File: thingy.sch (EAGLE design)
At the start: 20 parts, among them IC1 MCP6001T-I/OT, IC2 MAX9812LEXT+T, IC3 ESP-12, IC4 ADXL345BCCZ, J1 Interface, Q1 Electret Mic

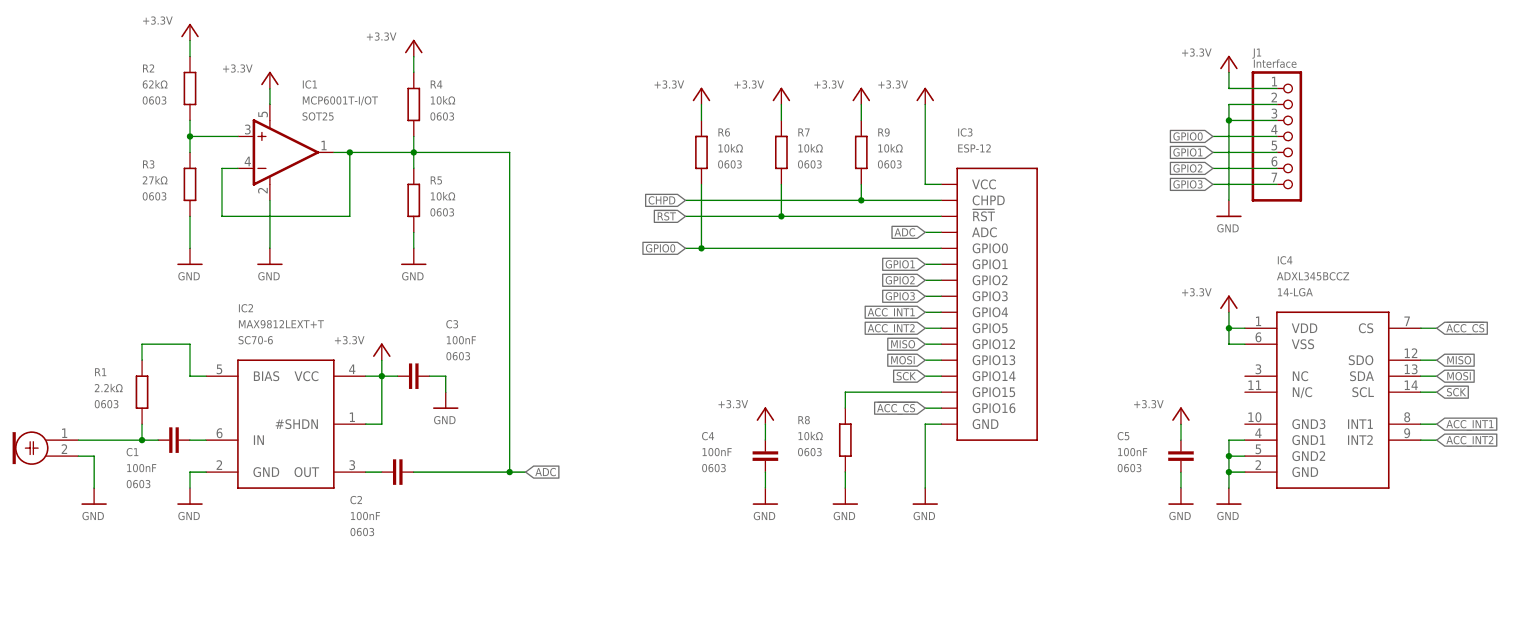
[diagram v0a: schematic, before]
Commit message: foo
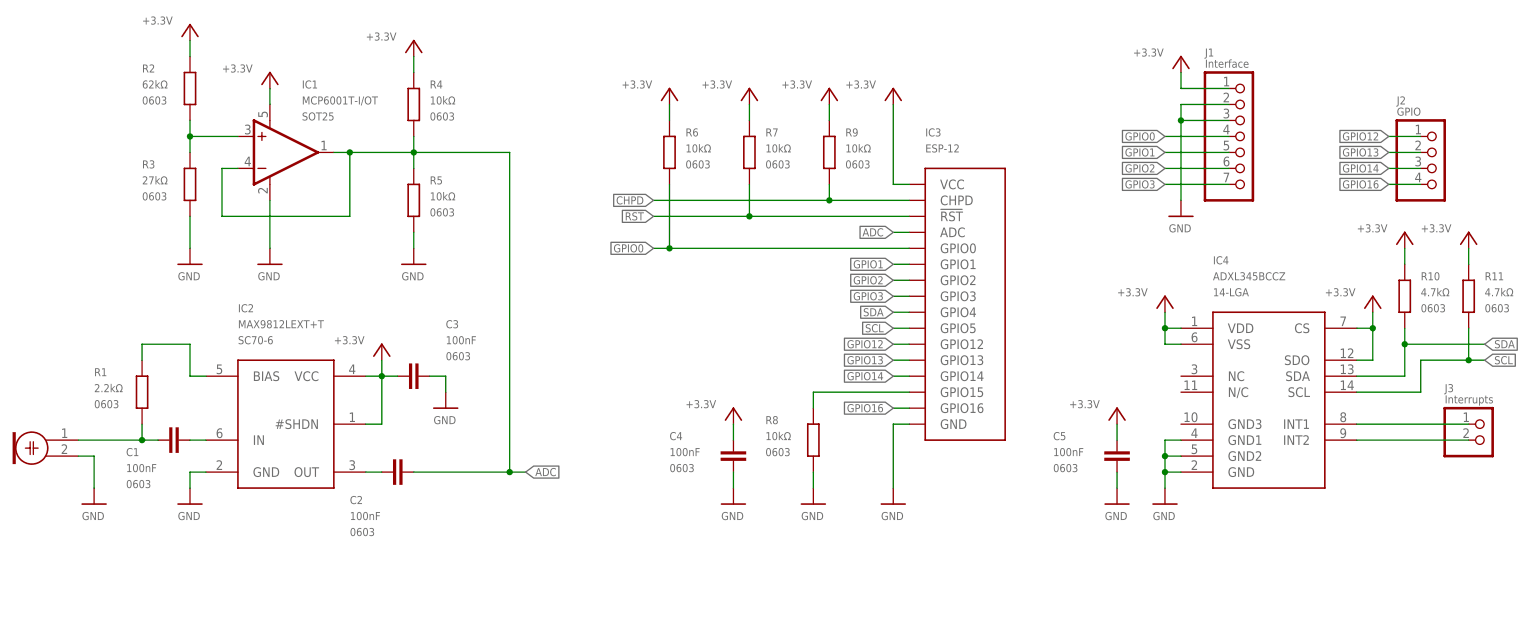
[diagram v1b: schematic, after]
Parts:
- added J2: GPIO, pinhead:PINHD-1X4
- added J3: Interrupts, pinhead:PINHD-1X2
- added R10, R11: 4.7kΩ, freetronics-luke:R0603
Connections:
- removed net !ACC_CS: IC3.GPIO16, IC4.CS
- removed net MISO: IC3.GPIO12, IC4.SDO
- removed net MOSI: IC3.GPIO13, IC4.SDA
- removed net SCK: IC3.GPIO14, IC4.SCL
- new net GPIO12: IC3.GPIO12, J2.1
- new net GPIO13: IC3.GPIO13, J2.2
- new net GPIO14: IC3.GPIO14, J2.3
- new net GPIO16: IC3.GPIO16, J2.4
- new net SCL: IC3.GPIO5, IC4.SCL, R11.1
- new net SDA: IC3.GPIO4, IC4.SDA, R10.1
- net +3.3V: now also IC4.CS, IC4.SDO, R10.2, R11.2
- net ACC_INT1: now also J3.1; no longer IC3.GPIO4
- net ACC_INT2: now also J3.2; no longer IC3.GPIO5
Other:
- note removed: "Could use I2C instead if you like."
- moved on the sheet: C4, C5, IC3, IC4, J1, R6, R7, R8, R9

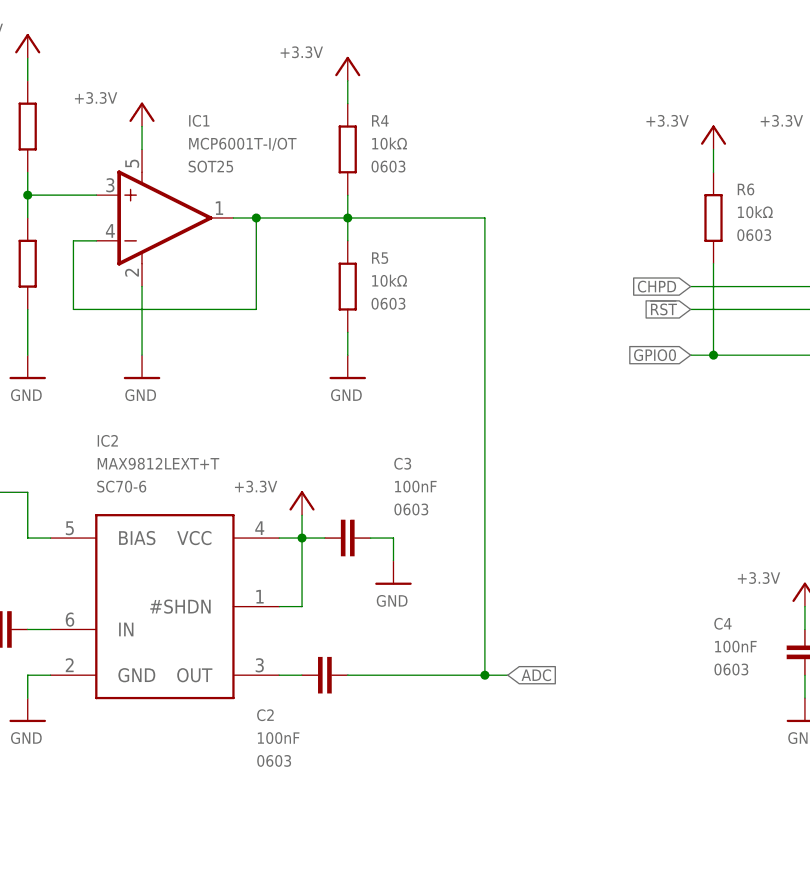
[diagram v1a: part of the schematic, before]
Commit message: foo
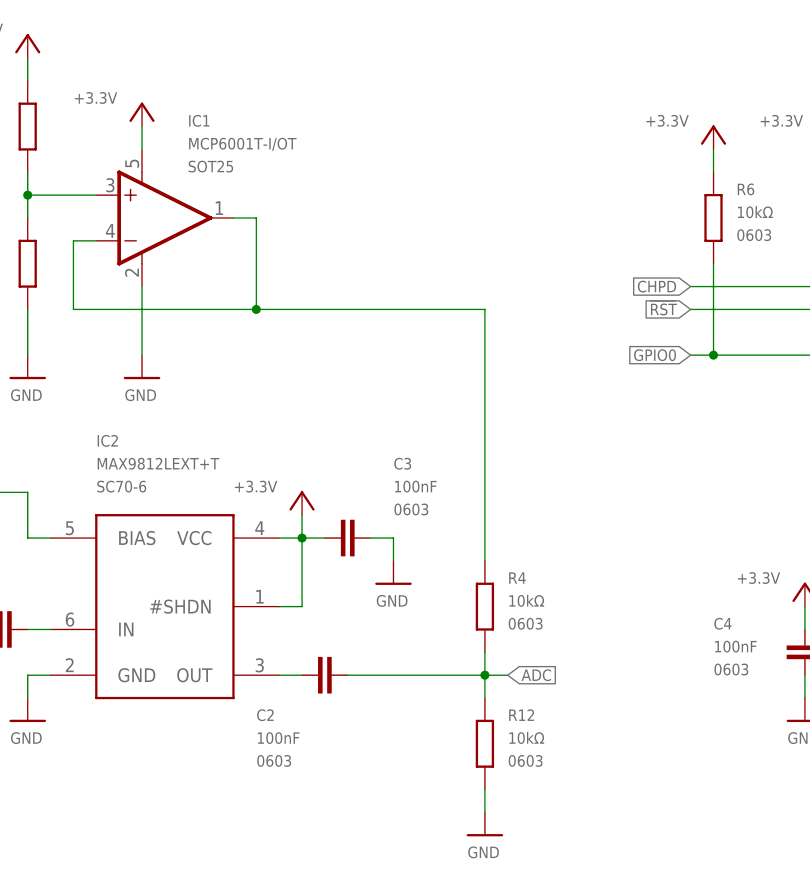
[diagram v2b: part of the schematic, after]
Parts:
- removed R5: 10kΩ, freetronics-luke:R0603
- added R12: 10kΩ, freetronics-luke:R0603
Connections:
- new net N$1: IC1.-IN, IC1.OUT, R4.2
- net +3.3V: no longer R4.2
- net ADC: now also R12.2; no longer IC1.-IN, IC1.OUT, R5.2
- net GND: now also R12.1; no longer R5.1
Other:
- moved on the sheet: R4
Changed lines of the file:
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@@
 <setting verticaltext="up"/>
 </settings>
-<grid distance="0.1" unitdist="inch" unit="inch" style="lines" multiple="1" display="no" altdistance="0.01" altunitdist="inch" altunit="inch"/>
+<grid distance="0.1" unitdist="inch" unit="inch" style="lines" multiple="1" display="yes" altdistance="0.01" altunitdist="inch" altunit="inch"/>
 <layers>
 <layer number="1" name="Top" color="4" fill="1" visible="no" active="no"/>
@@
 <part name="+3V9" library="supply1" deviceset="+3V3" device="" value="+3.3V"/>
 <part name="U$27" library="freetronics-luke" deviceset="GND" device=""/>
-<part name="+3V10" library="supply1" deviceset="+3V3" device="" value="+3.3V"/>
-<part name="U$29" library="freetronics-luke" deviceset="GND" device=""/>
 <part name="J1" library="pinhead" deviceset="PINHD-1X7" device="" value="Interface"/>
 <part name="+3V11" library="supply1" deviceset="+3V3" device="" value="+3.3V"/>
@@
 <attribute name="PACKAGE" value="0603"/>
 </part>
-<part name="R5" library="freetronics-luke" deviceset="R" device="0603" value="10kΩ">
-<attribute name="PACKAGE" value="0603"/>
-</part>
 <part name="R4" library="freetronics-luke" deviceset="R" device="0603" value="10kΩ">
 <attribute name="PACKAGE" value="0603"/>
@@
 <part name="+3V6" library="supply1" deviceset="+3V3" device="" value="+3.3V"/>
 <part name="+3V14" library="supply1" deviceset="+3V3" device="" value="+3.3V"/>
+<part name="R12" library="freetronics-luke" deviceset="R" device="0603" value="10kΩ">
+<attribute name="PACKAGE" value="0603"/>
+</part>
+<part name="U$1" library="freetronics-luke" deviceset="GND" device=""/>
 </parts>
 <sheets>
@@
 </instance>
 <instance part="U$27" gate="G$1" x="40.64" y="73.66" rot="MR0"/>
-<instance part="+3V10" gate="G$1" x="76.2" y="109.22" smashed="yes" rot="MR0">
-<attribute name="VALUE" x="68.58" y="109.22" size="1.27" layer="96"/>
-</instance>
-<instance part="U$29" gate="G$1" x="76.2" y="73.66" rot="MR0"/>
 <instance part="J1" gate="A" x="208.28" y="93.98" smashed="yes">
 <attribute name="NAME" x="201.93" y="106.68" size="1.27" layer="95"/>
@@
 <attribute name="VALUE" x="25.4" y="53.34" size="1.27" layer="96"/>
 </instance>
-<instance part="R5" gate="G$1" x="76.2" y="83.82" smashed="yes" rot="MR90">
-<attribute name="PACKAGE" x="78.74" y="81.28" size="1.27" layer="96"/>
-<attribute name="NAME" x="78.74" y="86.36" size="1.27" layer="95"/>
-<attribute name="VALUE" x="78.74" y="83.82" size="1.27" layer="96"/>
-</instance>
-<instance part="R4" gate="G$1" x="76.2" y="99.06" smashed="yes" rot="MR90">
-<attribute name="PACKAGE" x="78.74" y="96.52" size="1.27" layer="96"/>
-<attribute name="NAME" x="78.74" y="101.6" size="1.27" layer="95"/>
-<attribute name="VALUE" x="78.74" y="99.06" size="1.27" layer="96"/>
+<instance part="R4" gate="G$1" x="91.44" y="48.26" smashed="yes" rot="MR90">
+<attribute name="PACKAGE" x="93.98" y="45.72" size="1.27" layer="96"/>
+<attribute name="NAME" x="93.98" y="50.8" size="1.27" layer="95"/>
+<attribute name="VALUE" x="93.98" y="48.26" size="1.27" layer="96"/>
 </instance>
 <instance part="R6" gate="G$1" x="116.84" y="91.44" smashed="yes" rot="MR90">
@@
 <attribute name="VALUE" x="236.22" y="78.74" size="1.27" layer="96"/>
 </instance>
+<instance part="R12" gate="G$1" x="91.44" y="33.02" smashed="yes" rot="MR90">
+<attribute name="PACKAGE" x="93.98" y="30.48" size="1.27" layer="96"/>
+<attribute name="NAME" x="93.98" y="35.56" size="1.27" layer="95"/>
+<attribute name="VALUE" x="93.98" y="33.02" size="1.27" layer="96"/>
+</instance>
+<instance part="U$1" gate="G$1" x="91.44" y="22.86" rot="MR0"/>
 </instances>
 <busses>
@@
 </segment>
 <segment>
-<pinref part="U$29" gate="G$1" pin="GND"/>
-<wire x1="76.2" y1="76.2" x2="76.2" y2="78.74" width="0.1524" layer="91"/>
-<pinref part="R5" gate="G$1" pin="1"/>
-</segment>
-<segment>
 <pinref part="J1" gate="A" pin="2"/>
 <wire x1="205.74" y1="99.06" x2="198.12" y2="99.06" width="0.1524" layer="91"/>
@@
 <pinref part="U$28" gate="G$1" pin="GND"/>
 <junction x="198.12" y="96.52"/>
+</segment>
+<segment>
+<pinref part="R12" gate="G$1" pin="1"/>
+<pinref part="U$1" gate="G$1" pin="GND"/>
+<wire x1="91.44" y1="25.4" x2="91.44" y2="27.94" width="0.1524" layer="91"/>
 </segment>
 </net>
@@
 </segment>
 <segment>
-<pinref part="+3V10" gate="G$1" pin="+3V3"/>
-<wire x1="76.2" y1="106.68" x2="76.2" y2="104.14" width="0.1524" layer="91"/>
-<pinref part="R4" gate="G$1" pin="2"/>
-</segment>
-<segment>
 <pinref part="J1" gate="A" pin="1"/>
 <wire x1="205.74" y1="101.6" x2="198.12" y2="101.6" width="0.1524" layer="91"/>
@@
 </segment>
 <segment>
-<pinref part="IC1" gate="G$1" pin="-IN"/>
-<wire x1="48.26" y1="88.9" x2="45.72" y2="88.9" width="0.1524" layer="91"/>
-<wire x1="45.72" y1="88.9" x2="45.72" y2="81.28" width="0.1524" layer="91"/>
-<wire x1="45.72" y1="81.28" x2="66.04" y2="81.28" width="0.1524" layer="91"/>
-<wire x1="66.04" y1="81.28" x2="66.04" y2="91.44" width="0.1524" layer="91"/>
-<pinref part="IC1" gate="G$1" pin="OUT"/>
-<wire x1="66.04" y1="91.44" x2="63.5" y2="91.44" width="0.1524" layer="91"/>
 <pinref part="C2" gate="G$1" pin="2"/>
 <wire x1="76.2" y1="40.64" x2="91.44" y2="40.64" width="0.1524" layer="91"/>
-<wire x1="91.44" y1="40.64" x2="91.44" y2="91.44" width="0.1524" layer="91"/>
-<wire x1="91.44" y1="91.44" x2="76.2" y2="91.44" width="0.1524" layer="91"/>
-<junction x="66.04" y="91.44"/>
-<wire x1="76.2" y1="91.44" x2="66.04" y2="91.44" width="0.1524" layer="91"/>
-<wire x1="76.2" y1="93.98" x2="76.2" y2="91.44" width="0.1524" layer="91"/>
-<junction x="76.2" y="91.44"/>
-<wire x1="76.2" y1="88.9" x2="76.2" y2="91.44" width="0.1524" layer="91"/>
+<wire x1="91.44" y1="40.64" x2="91.44" y2="43.18" width="0.1524" layer="91"/>
 <wire x1="91.44" y1="40.64" x2="93.98" y2="40.64" width="0.1524" layer="91"/>
 <label x="93.98" y="40.64" size="1.27" layer="95" xref="yes"/>
 <junction x="91.44" y="40.64"/>
-<pinref part="R5" gate="G$1" pin="2"/>
 <pinref part="R4" gate="G$1" pin="1"/>
+<pinref part="R12" gate="G$1" pin="2"/>
+<wire x1="91.44" y1="38.1" x2="91.44" y2="40.64" width="0.1524" layer="91"/>
 </segment>
 </net>
@@
 </segment>
 </net>
+<net name="N$1" class="0">
+<segment>
+<pinref part="IC1" gate="G$1" pin="OUT"/>
+<wire x1="66.04" y1="91.44" x2="63.5" y2="91.44" width="0.1524" layer="91"/>
+<pinref part="IC1" gate="G$1" pin="-IN"/>
+<wire x1="48.26" y1="88.9" x2="45.72" y2="88.9" width="0.1524" layer="91"/>
+<wire x1="45.72" y1="88.9" x2="45.72" y2="81.28" width="0.1524" layer="91"/>
+<wire x1="45.72" y1="81.28" x2="66.04" y2="81.28" width="0.1524" layer="91"/>
+<wire x1="66.04" y1="91.44" x2="66.04" y2="81.28" width="0.1524" layer="91"/>
+<wire x1="66.04" y1="81.28" x2="91.44" y2="81.28" width="0.1524" layer="91"/>
+<wire x1="91.44" y1="81.28" x2="91.44" y2="53.34" width="0.1524" layer="91"/>
+<pinref part="R4" gate="G$1" pin="2"/>
+<junction x="66.04" y="81.28"/>
+</segment>
+</net>
